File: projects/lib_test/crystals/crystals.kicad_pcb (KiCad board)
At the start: 2 copper layers, 80 x 60 mm, 0 parts

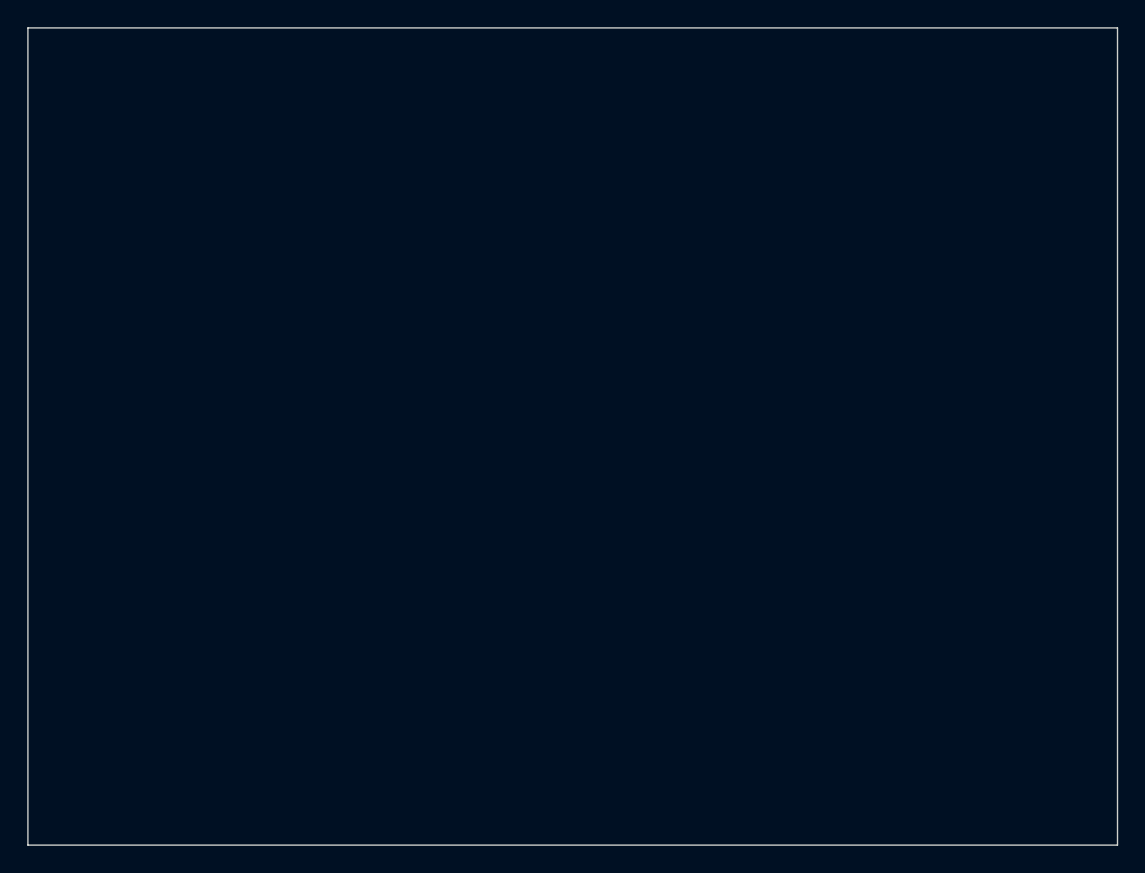
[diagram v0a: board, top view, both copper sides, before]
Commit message: updated crystals test project
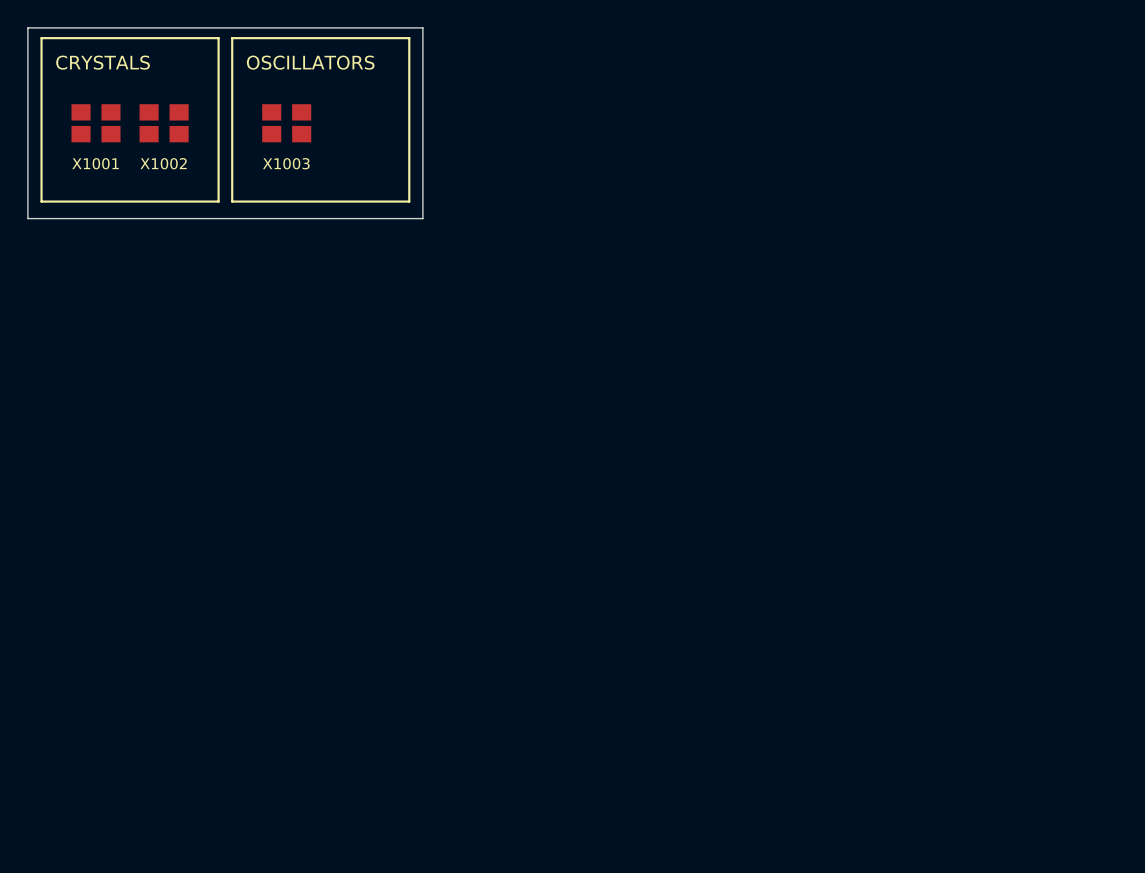
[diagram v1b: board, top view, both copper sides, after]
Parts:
- added X1001: 12MHz, lily_footprints:crystal_3225, F.Cu at (115.0, 77.0)
- added X1002: 16MHz, lily_footprints:crystal_3225, F.Cu at (120.0, 77.0)
- added X1003: 50MHz, lily_footprints:crystal_3225, F.Cu at (129.0, 77.0)
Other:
- board size 80 x 60 mm -> 29 x 14 mm
- board text added: "CRYSTALS"
- board text added: "OSCILLATORS"
